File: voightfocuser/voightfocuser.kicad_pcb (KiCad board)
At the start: 2 copper layers, 69.9 x 47.2 mm, 58 parts, among them J1 Barrel_Jack, J2 USB_B_Micro, J3 Programming Header, M1 Stepper_Motor_bipolar, SW1 SW_Push, SW2 SW_SPDT, SW3 Limit Switch, SW4 Rotary_Encoder_Switch, SW5 SP5T, U1 FT230XS, U2 TXB0104D, U3 DRV8825, U4 ATmega328P-AU, U5 DHT11, Y1 16MHz

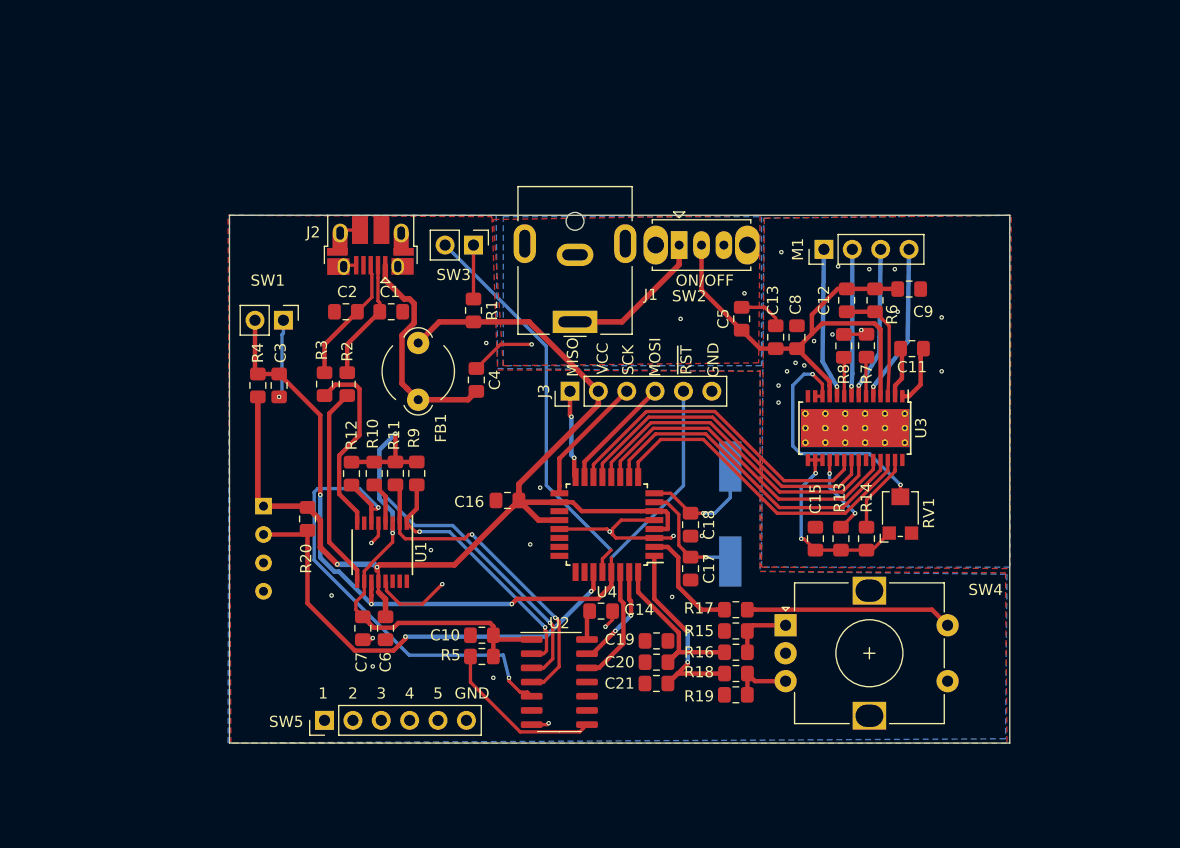
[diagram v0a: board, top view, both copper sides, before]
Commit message: bigger board. routing prototype finished?
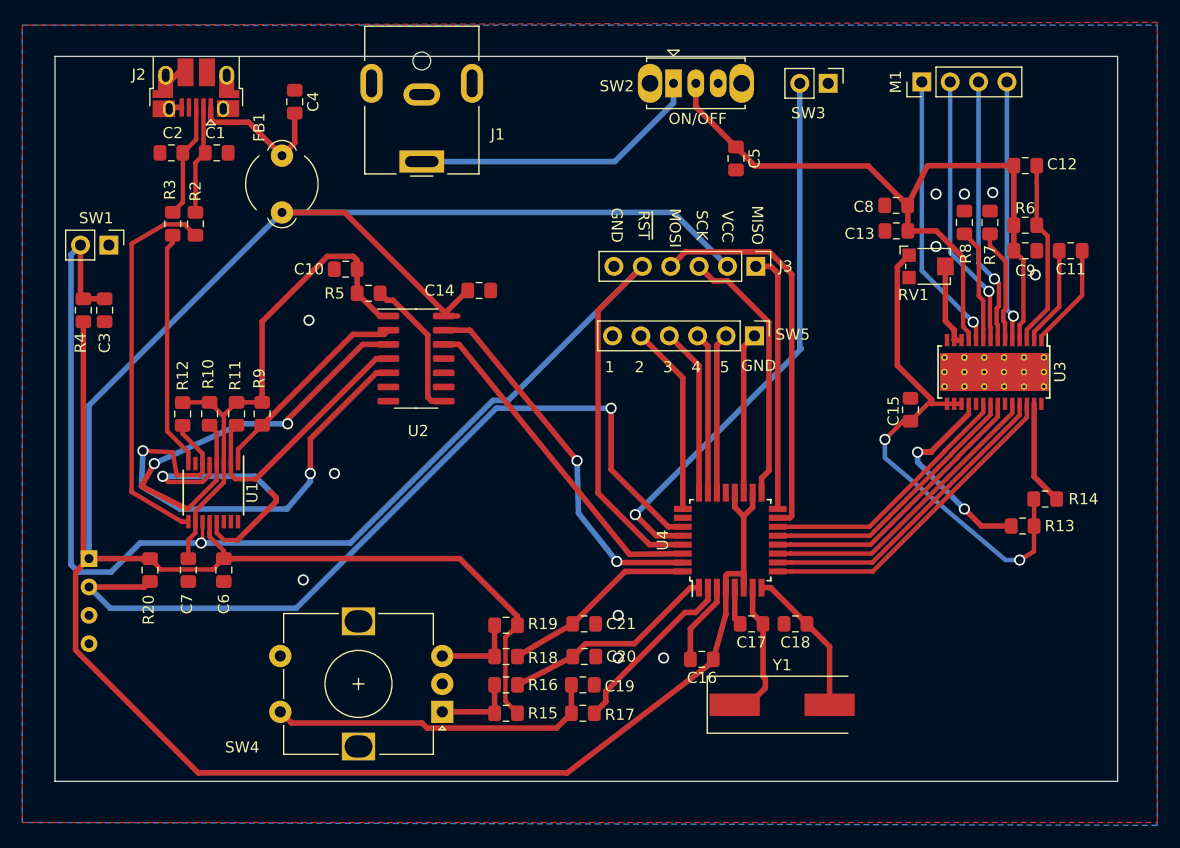
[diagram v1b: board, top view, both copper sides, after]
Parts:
- removed R1: 10k, Resistor_SMD:R_0805_2012Metric_Pad1.15x1.40mm_HandSolder
- Y1: moved to F.Cu
- moved SW5 51.6 mm to (167.8, 88.8), turned to 270 degrees
- moved C10 35.0 mm to (131.2, 82.8)
- moved SW3 34.9 mm to (174.4, 66.2)
- moved R5 34.1 mm to (133.2, 85.0), turned to 180 degrees
- moved SW4 31.7 mm to (139.8, 122.4), turned to 180 degrees
- moved U2 31.7 mm to (137.5, 90.8)
- moved C14 30.7 mm to (143.1, 84.7)
- moved C4 29.7 mm to (126.6, 67.8)
- moved C16 22.5 mm to (163.1, 117.7)
- moved RV1 22.2 mm to (183.4, 82.5), turned to 0 degrees
- moved R15 21.9 mm to (145.5, 122.6), turned to 0 degrees
- moved R19 21.5 mm to (145.5, 114.7), turned to 180 degrees
- moved C1 21.1 mm to (119.6, 72.4)
- moved C2 21.1 mm to (115.6, 72.4)
- moved J2 21.1 mm to (117.8, 66.6)
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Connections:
- net Net-(C17-Pad2) renamed XTAL_N
- net Net-(C18-Pad2) renamed XTAL_P
- C20 pad 2: INT0 -> INT1
- C21 pad 1: INT1 -> INT0
- R16 pad 2: INT0 -> INT1
- R18 pad 2: INT1 -> INT0
- SW3 pad 1: Net-(R1-Pad1) -> GND
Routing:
- net VCC: track 99.4 -> 274.9 mm, vias 2 -> 0
- net ~RESET: track 75.4 -> 159.7 mm, vias 6 -> 1
- net TEMP: track 41.9 -> 74.6 mm, vias 2 -> 1
- net V3P3OUT: track 17.8 -> 46.4 mm
- net MOSI: track 10.3 -> 35.2 mm
- net TX: track 9.30 -> 33.6 mm
- net VDD12+: track 45.2 -> 68.4 mm
- net RX: track 10.7 -> 30.4 mm
- net HIGH: track 0.00 -> 17.0 mm
- net Net-(R2-Pad1): track 18.3 -> 34.6 mm
- net MISO: track 7.90 -> 23.3 mm, vias 2 -> 0
- net Net-(RV1-Pad2): track 22.8 -> 7.58 mm, vias 2 -> 0
- net MEDHIGH: track 0.00 -> 15.1 mm
- net LOW: track 0.00 -> 14.4 mm
- net MED: track 0.00 -> 14.4 mm
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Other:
- board size 69.9 x 47.2 mm -> 95.1 x 64.9 mm
- net class Default: via_dia 0.000686 -> 0.8; via_drill 0.00033 -> 0.6
- net class Power: via_dia 0.1 -> 1; via_drill 0.05 -> 0.8
- net class Stepper removed
